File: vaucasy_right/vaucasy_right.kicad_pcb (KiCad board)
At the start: 2 copper layers, 153.2 x 136.5 mm, 105 parts, among them J1 USB_C, J2 OLED_128x32, J4 Trackball, J5 HC-05 BT, J6 DEBUG, SW1 SW_SPDT, SW2 SW_Push, SW3 RotaryEncoder_Switch, U1 STM32F401RET6, U2 USBLC6-2SC6, U3 XC6206, U4 TRRS, Y1 8MHz

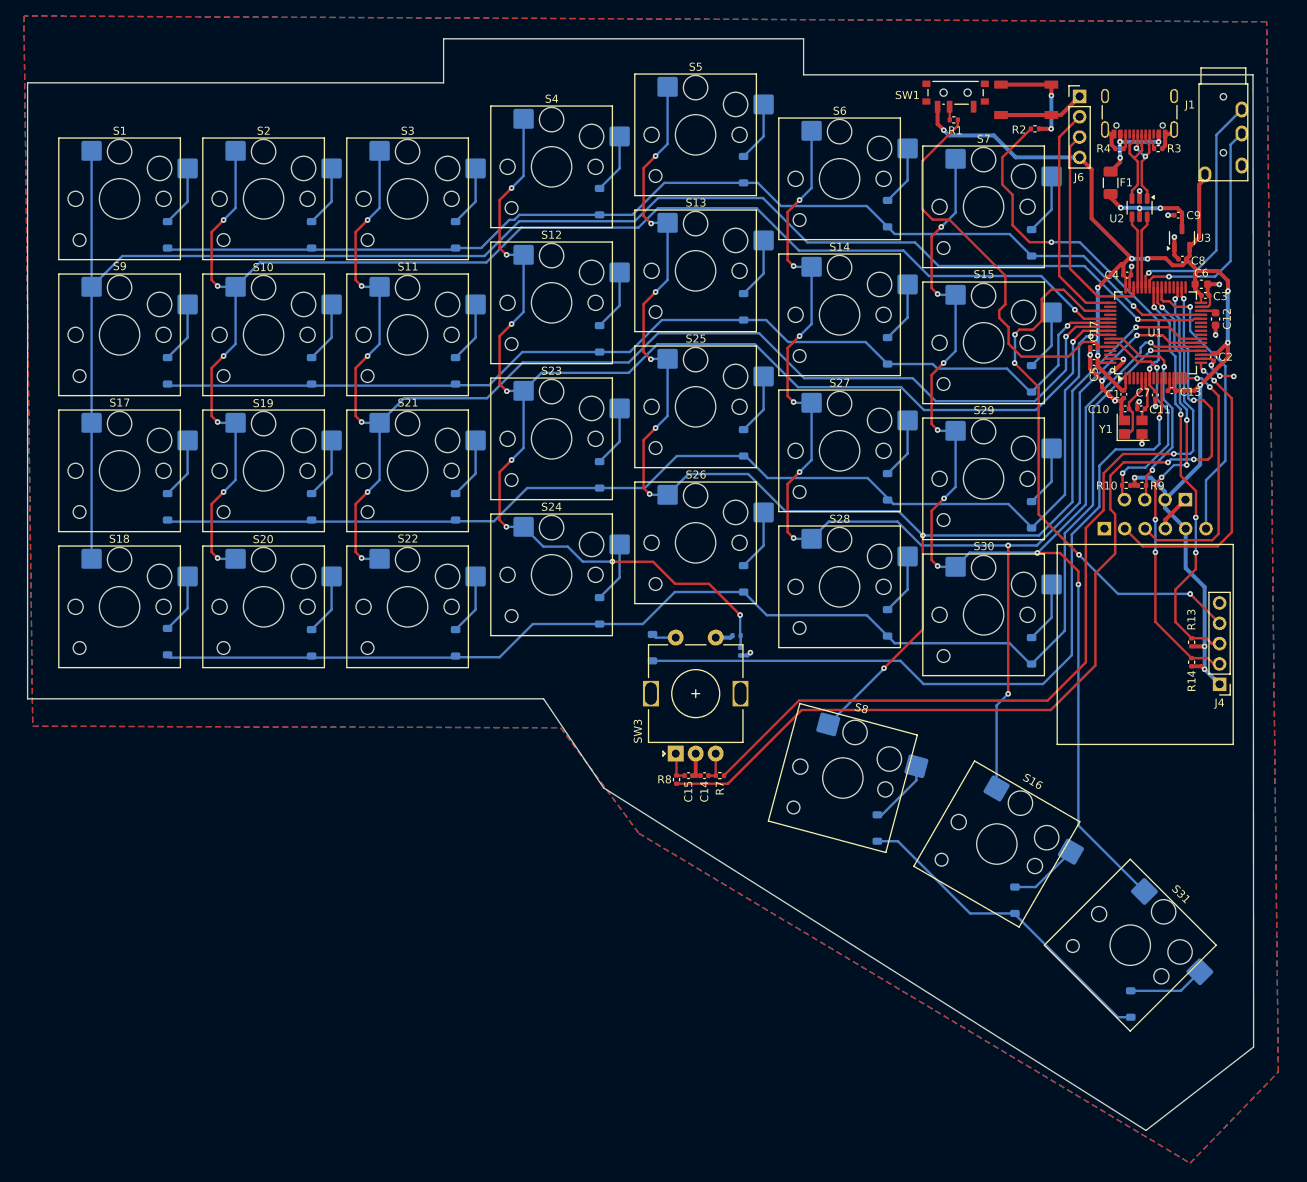
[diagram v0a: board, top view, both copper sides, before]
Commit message: ordered
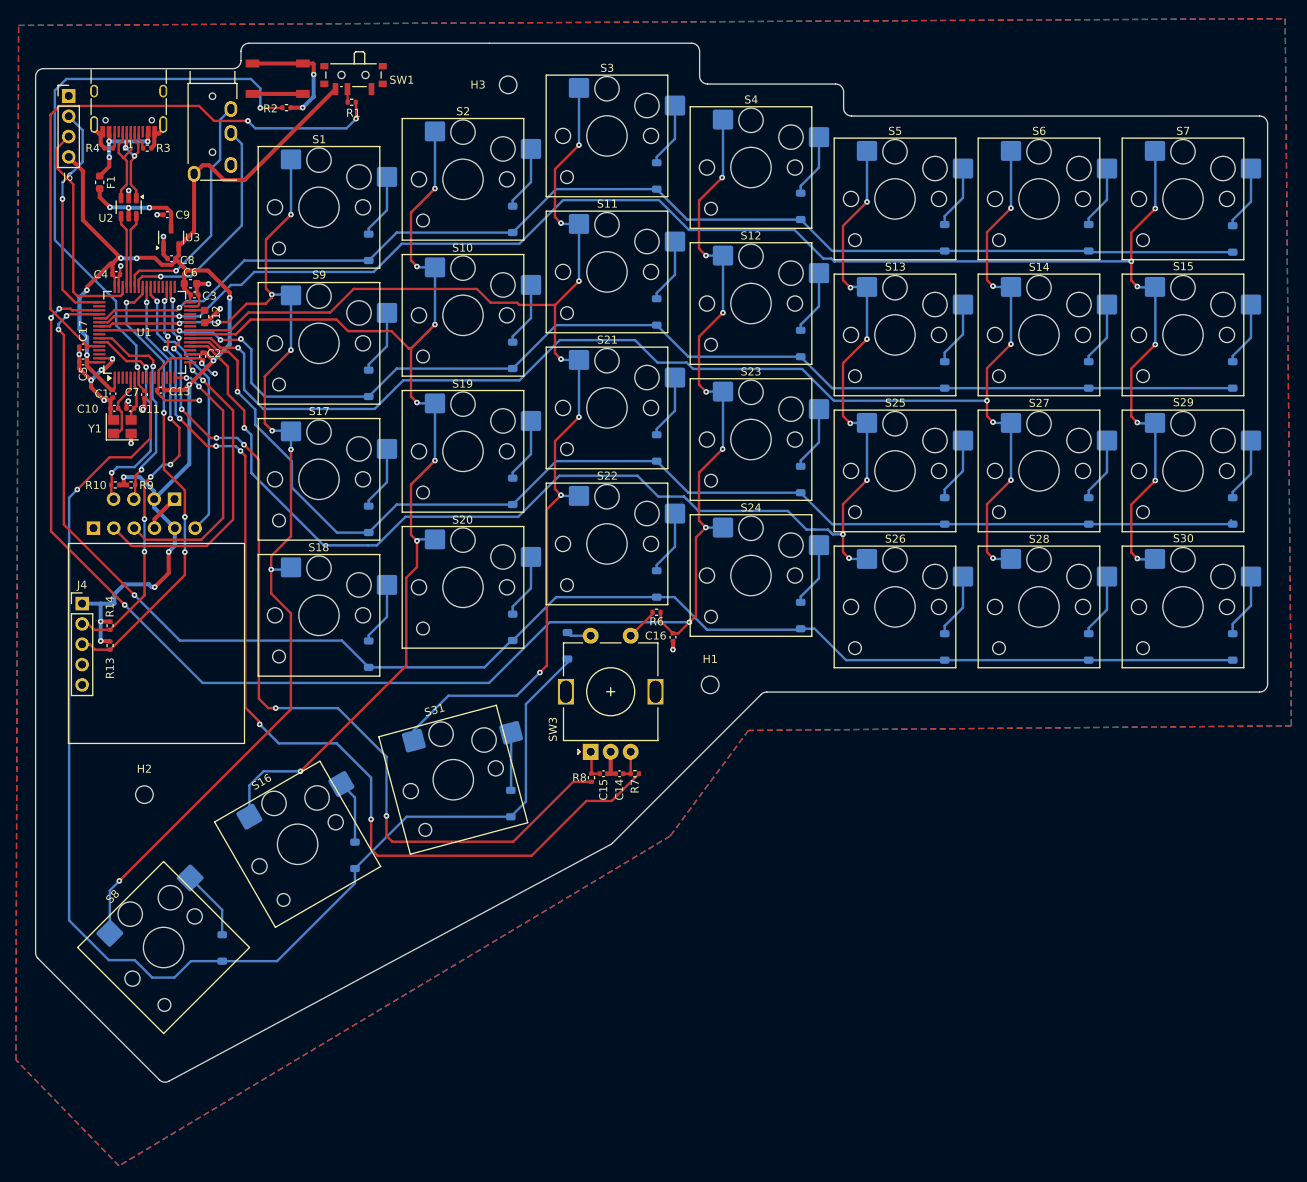
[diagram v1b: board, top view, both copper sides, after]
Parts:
- added H1: MountingHole, MountingHole:MountingHole_2.2mm_M2, F.Cu at (109.3, 108.1)
- added H2: MountingHole, MountingHole:MountingHole_2.2mm_M2, F.Cu at (38.6, 121.8)
- added H3: MountingHole, MountingHole:MountingHole_2.2mm_M2, F.Cu at (84.1, 33.1)
- C16, R6: moved to F.Cu
- F1: footprint Fuse:Fuse_1206_3216Metric -> Fuse:Fuse_0603_1608Metric
- J1: footprint Connector_USB:USB_C_Receptacle_GCT_USB4105-xx-A_16P_TopMnt_Horizontal -> Connector_USB:USB_C_Receptacle_HRO_TYPE-C-31-M-12
- J5: footprint Connector_PinSocket_2.54mm:PinSocket_1x06_P2.54mm_Horizontal -> Connector_PinSocket_2.54mm:PinSocket_1x06_P2.54mm_Vertical
- moved J4 142.5 mm to (30.8, 97.9), turned to 0 degrees
- moved R14 135.3 mm to (34.3, 100.7), turned to -90 degrees
- moved R13 135.2 mm to (34.3, 103.2), turned to 90 degrees
- moved J1 126.4 mm to (36.6, 34.9)
- moved C12 126.4 mm to (46.1, 62.1)
- moved C1 126.4 mm to (34.7, 71.7)
- moved C13 126.4 mm to (40.7, 71.3)
- moved C17 126.4 mm to (30.9, 65.9)
- moved C5 126.4 mm to (30.9, 67.7)
- moved J2 126.4 mm to (32.6, 86.5)
- moved R9 126.4 mm to (36.9, 83.1)
- moved U3 126.4 mm to (41.9, 52.2)
- moved C2 126.4 mm to (45.9, 67.1)
- moved C3 126.4 mm to (44.9, 59.4)
- moved C6 126.4 mm to (44.4, 58.0)
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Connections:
- D16 pad 1: LROW4 -> LRow 4
- D31 pad 1: LROW4 -> LRow 4
- D8 pad 1: LROW4 -> LRow 4
- J4 pad 4: LTRACK_INT -> unconnected-(J4-INT-Pad4)
- S16 pad 1: LColumn 5 -> LColumn 1
- S31 pad 1: LColumn 6 -> LColumn 2
- S8 pad 1: LColumn 4 -> LColumn 0
- U1 pad 20: LRow 3 -> unconnected-(U1-PA4-Pad20)
- U1 pad 21: LColumn 6 -> LColumn 4
- U1 pad 22: LColumn 5 -> LRow 2
- U1 pad 23: LColumn 4 -> LColumn 5
- U1 pad 24: unconnected-(U1-PC4-Pad24) -> LColumn 1
- U1 pad 25: unconnected-(U1-PC5-Pad25) -> LColumn 2
- U1 pad 28: LColumn 0 -> unconnected-(U1-PB2-Pad28)
- U1 pad 29: LRow 0 -> unconnected-(U1-PB10-Pad29)
- U1 pad 51: LTRACK_INT -> LColumn 3
- U1 pad 52: unconnected-(U1-PC11-Pad52) -> LRow 3
- U1 pad 53: LColumn 1 -> LRow 0
- U1 pad 54: LRow 1 -> LColumn 6
- U1 pad 55: LColumn 2 -> LColumn 0
- U1 pad 56: LColumn 3 -> LRow 1
- U1 pad 57: LRow 2 -> unconnected-(U1-PB5-Pad57)
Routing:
- net LTRACK_INT: track 68.9 -> 0.00 mm, vias 4 -> 0
- net LRow 4: track 97.2 -> 163.9 mm
- net LColumn 0: track 200.7 -> 142.2 mm, vias 1 -> 9
- net LColumn 1: track 181.1 -> 138.0 mm
- net LROW4: track 40.8 -> 0.00 mm
- net LColumn 6: track 161.3 -> 200.3 mm, vias 9 -> 8
- net LNRST: track 46.9 -> 74.1 mm
- net LRow 3: track 167.1 -> 191.4 mm, vias 1 -> 3
- net LBOOT0: track 50.8 -> 74.9 mm, vias 0 -> 2
- net LRow 1: track 131.0 -> 154.6 mm, vias 1 -> 3
- net LColumn 3: track 183.6 -> 204.9 mm, vias 9 -> 10
- net LENCODER_B: track 109.5 -> 125.7 mm, vias 2 -> 8
- net LColumn 4: track 181.3 -> 166.9 mm, vias 9 -> 8
- net LColumn 2: track 167.6 -> 153.7 mm
- net LRow 0: track 139.6 -> 151.6 mm
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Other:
- board size 153.2 x 136.5 mm -> 154 x 129.9 mm
